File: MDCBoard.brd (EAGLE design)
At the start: 43.9 x 32.6 mm, 200 parts, among them J1 JUMPER-SOLDER, J10 MICROSD-SOCKET, J11 USB-C-RECEPTACLE-KOREANHRO, J2 JUMPER-SOLDER, J3 JUMPER-SOLDER, J4 JUMPER-SOLDER, J5 JST-SM02B-SRSS-TB, J6 JUMPER-SOLDER, J7 JUMPER-SOLDER, J8 JUMPER-SOLDER, Q1 PMOS-NEXPERIA-SOT1220, Q2 PMOS-NEXPERIA-SOT1220, Q3 PMOS-NEXPERIA-SOT1220, Q4 DIODESINC-DMG2305UX, Q5 DIODESINC-DMG2305UX, Q6 DIODESINC-DMG2305UX, Q7 DIODESINC-DMG2305UX, Q8 DIODESINC-DMG2305UX, U1 TI-TPS2116, U10 TI-TPS22919DCK, U11 TI-TPS22919DCK, U12 TI-TPS22919DCK, U13 TI-TPS22919DCK, U14 TI-MSP430FR2422IRHL, U16 TI-TXB0102, U17 PANASONIC-EKMB110711X, U18 LATTICE-ICE40HX4K-BG121, U19 WINBOND-W25Q40EW, U2 DIODESINC-AP7350, U20 NEXPERIA-74LVC1G98-OR-INV-INP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, U21 NEXPERIA-74LVC1G98-BUFFER, U22 ON-AR0330CS1C12SPKA0, U23 ALLIANCE-AS4C8M16MSA-6BIN, U24 STM-STM32F730, U25 DIODESINC-DT1446-04V-7, U26 NEXPERIA-74LVC1G98-INVERTER, U3 NEXPERIA-74LVC1G98-NOR, U4 MICROCHIP-MCP7383X, U5 NEXPERIA-74LVC1G98-INVERTER, U6 EATON-STN101, U7 TI-TPS62A01, U8 TI-TPS62A01, U9 TI-TPS62A01, X1 EPSON-FC-135, X2 SITIME-SIT8021, X3 SITIME-SIT8021

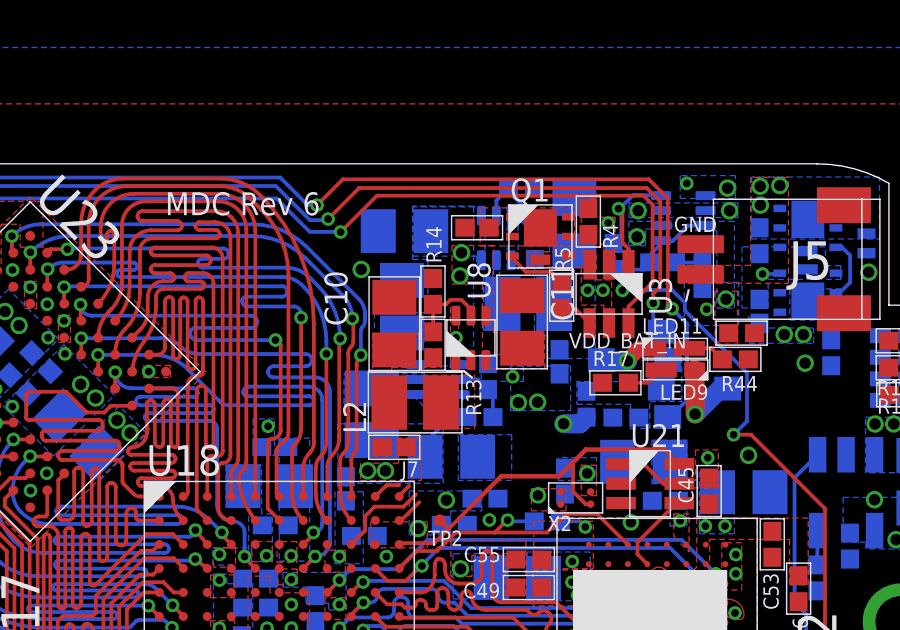
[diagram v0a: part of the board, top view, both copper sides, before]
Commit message: 15 airwires
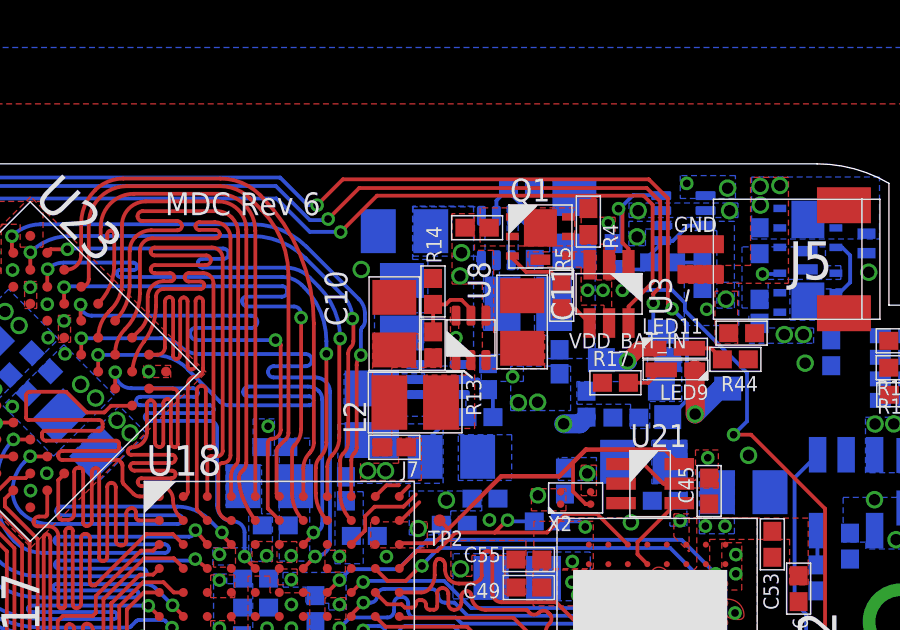
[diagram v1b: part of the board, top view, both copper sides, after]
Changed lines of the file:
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@@
 <grid distance="10" unitdist="mil" unit="mil" style="lines" multiple="1" display="no" altdistance="0.00254" altunitdist="mm" altunit="mil"/>
 <layers>
-<layer number="1" name="Top" color="4" fill="1" visible="no" active="yes"/>
+<layer number="1" name="Top" color="4" fill="1" visible="yes" active="yes"/>
 <layer number="2" name="Ground" color="16" fill="1" visible="no" active="yes"/>
 <layer number="3" name="Route3" color="17" fill="1" visible="no" active="no"/>
@@
 <layer number="13" name="Route13" color="21" fill="1" visible="no" active="no"/>
 <layer number="14" name="Route14" color="22" fill="1" visible="no" active="no"/>
-<layer number="15" name="Power" color="42" fill="1" visible="yes" active="yes"/>
+<layer number="15" name="Power" color="42" fill="1" visible="no" active="yes"/>
 <layer number="16" name="Bottom" color="1" fill="1" visible="no" active="yes"/>
-<layer number="17" name="Pads" color="2" fill="1" visible="no" active="yes"/>
+<layer number="17" name="Pads" color="2" fill="1" visible="yes" active="yes"/>
 <layer number="18" name="Vias" color="2" fill="1" visible="yes" active="yes"/>
 <layer number="19" name="Unrouted" color="6" fill="1" visible="no" active="yes"/>
-<layer number="20" name="Dimension" color="24" fill="1" visible="no" active="yes"/>
-<layer number="21" name="tPlace" color="7" fill="1" visible="no" active="yes"/>
+<layer number="20" name="Dimension" color="24" fill="1" visible="yes" active="yes"/>
+<layer number="21" name="tPlace" color="7" fill="1" visible="yes" active="yes"/>
 <layer number="22" name="bPlace" color="7" fill="1" visible="no" active="yes"/>
-<layer number="23" name="tOrigins" color="15" fill="1" visible="no" active="yes"/>
+<layer number="23" name="tOrigins" color="15" fill="1" visible="yes" active="yes"/>
 <layer number="24" name="bOrigins" color="15" fill="1" visible="no" active="yes"/>
-<layer number="25" name="tNames" color="7" fill="1" visible="no" active="yes"/>
+<layer number="25" name="tNames" color="7" fill="1" visible="yes" active="yes"/>
 <layer number="26" name="bNames" color="7" fill="1" visible="no" active="yes"/>
-<layer number="27" name="tValues" color="7" fill="1" visible="no" active="yes"/>
+<layer number="27" name="tValues" color="7" fill="1" visible="yes" active="yes"/>
 <layer number="28" name="bValues" color="7" fill="1" visible="no" active="yes"/>
-<layer number="29" name="tStop" color="7" fill="3" visible="no" active="yes"/>
+<layer number="29" name="tStop" color="7" fill="3" visible="yes" active="yes"/>
 <layer number="30" name="bStop" color="7" fill="6" visible="no" active="yes"/>
-<layer number="31" name="tCream" color="7" fill="4" visible="no" active="yes"/>
+<layer number="31" name="tCream" color="7" fill="4" visible="yes" active="yes"/>
 <layer number="32" name="bCream" color="7" fill="5" visible="no" active="yes"/>
-<layer number="33" name="tFinish" color="6" fill="3" visible="no" active="yes"/>
+<layer number="33" name="tFinish" color="6" fill="3" visible="yes" active="yes"/>
 <layer number="34" name="bFinish" color="6" fill="6" visible="no" active="yes"/>
-<layer number="35" name="tGlue" color="7" fill="4" visible="no" active="yes"/>
+<layer number="35" name="tGlue" color="7" fill="4" visible="yes" active="yes"/>
 <layer number="36" name="bGlue" color="7" fill="5" visible="no" active="yes"/>
-<layer number="37" name="tTest" color="7" fill="1" visible="no" active="yes"/>
+<layer number="37" name="tTest" color="7" fill="1" visible="yes" active="yes"/>
 <layer number="38" name="bTest" color="7" fill="1" visible="no" active="yes"/>
-<layer number="39" name="tKeepout" color="4" fill="11" visible="no" active="yes"/>
+<layer number="39" name="tKeepout" color="4" fill="11" visible="yes" active="yes"/>
 <layer number="40" name="bKeepout" color="1" fill="11" visible="no" active="yes"/>
-<layer number="41" name="tRestrict" color="4" fill="10" visible="no" active="yes"/>
+<layer number="41" name="tRestrict" color="4" fill="10" visible="yes" active="yes"/>
 <layer number="42" name="bRestrict" color="1" fill="10" visible="no" active="yes"/>
 <layer number="43" name="vRestrict" color="2" fill="10" visible="no" active="yes"/>
@@
 <contactref element="U7" pad="4"/>
 <polygon width="0.127" layer="1" thermals="no">
-<vertex x="28.322021875" y="29.92628125"/>
-<vertex x="26.93771875" y="29.92628125"/>
+<vertex x="28.322021875" y="29.766259375"/>
+<vertex x="27.686" y="29.766259375"/>
+<vertex x="27.686" y="30.988"/>
+<vertex x="26.924" y="30.988"/>
+<vertex x="26.93771875" y="30.97428125"/>
 <vertex x="26.93771875" y="28.64358125"/>
 <vertex x="27.948640625" y="28.64358125"/>
@@
 <vertex x="27.654" y="31.242"/>
 </polygon>
-<wire x1="27.916" y1="30.917740625" x2="27.372425" y2="30.522221875" width="0" layer="19" extent="1-16"/>
 </signal>
 <signal name="VDD_B_1V8">
@@
 <vertex x="25.416259375" y="25.0825"/>
 <vertex x="27.4" y="25.0825"/>
-<vertex x="27.4" y="24.892"/>
-<vertex x="26.8437375" y="24.3357375"/>
-<vertex x="26.226521875" y="24.3357375"/>
-<vertex x="25.73121875" y="24.831040625"/>
-<vertex x="25.416259375" y="24.831040625"/>
+<vertex x="27.4" y="24.235509375"/>
+<vertex x="25.416259375" y="24.235509375"/>
 </polygon>
 <polygon width="0.127" layer="1" thermals="no">
